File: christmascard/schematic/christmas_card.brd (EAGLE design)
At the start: 50 x 50 mm, 70 parts, among them IC1 WS2811-SOP8, IC2 WS2811-SOP8, IC5 WS2811-SOP8, IC7 74LS595D, U3 ATTINY24/44/84-SSU, X2 USB-MICROB

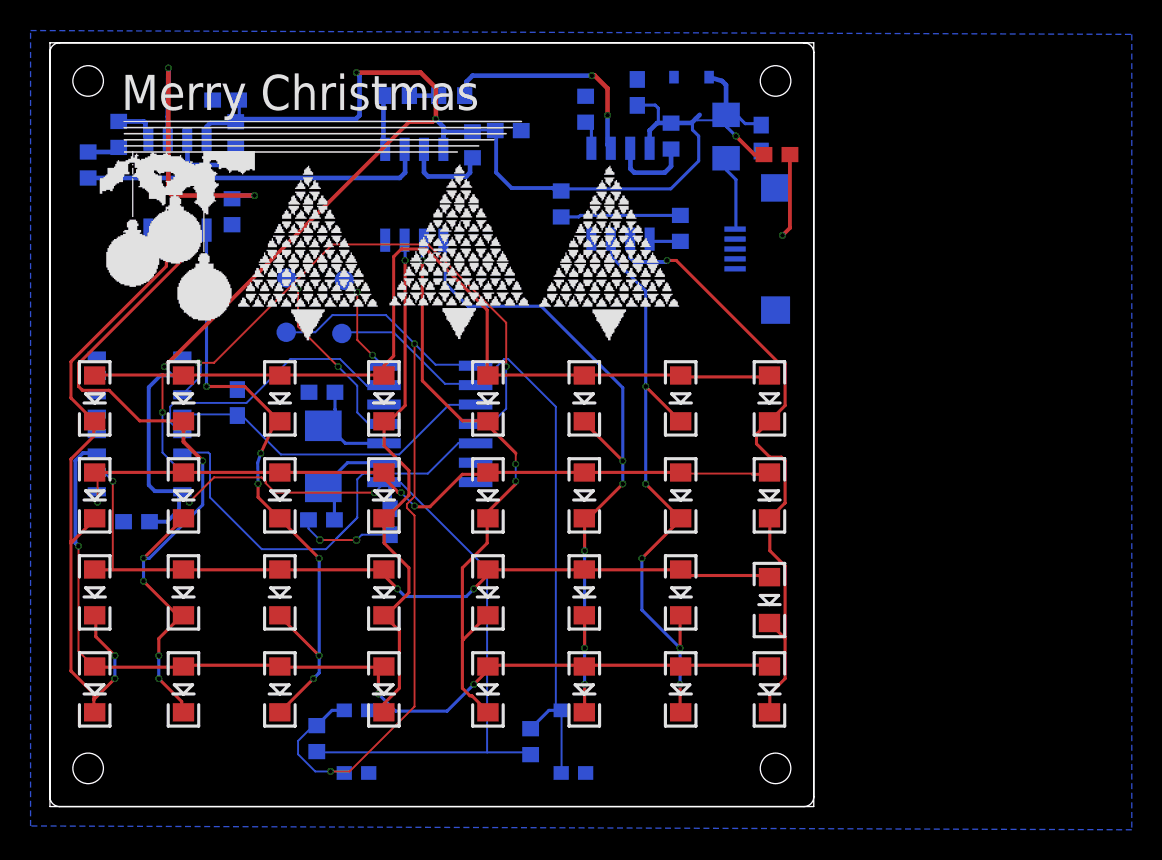
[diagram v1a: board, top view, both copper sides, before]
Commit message: Removed unused files, update board, code and other changes
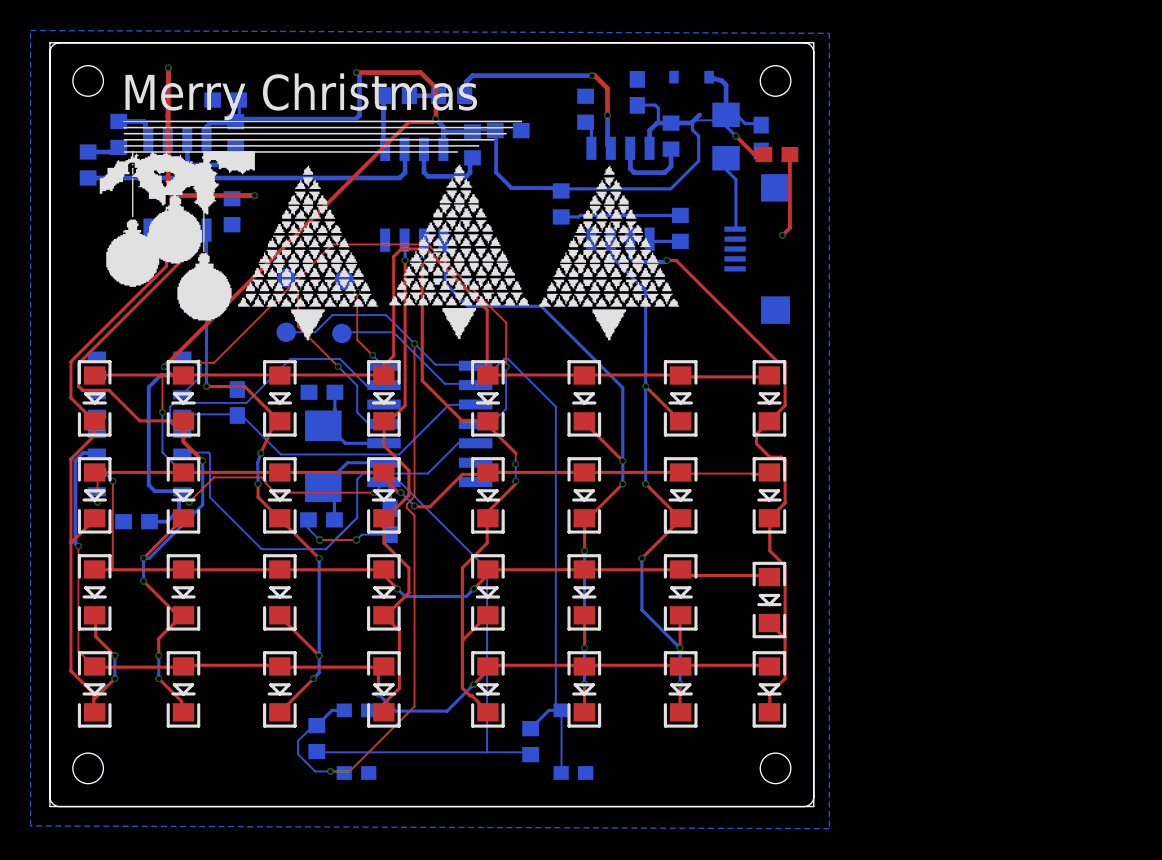
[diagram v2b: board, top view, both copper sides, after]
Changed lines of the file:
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@@
 <drawing>
 <settings>
-<setting alwaysvectorfont="yes"/>
+<setting alwaysvectorfont="no"/>
 <setting keepoldvectorfont="yes"/>
 <setting verticaltext="up"/>
@@
 <polygon width="0.254" layer="16">
 <vertex x="-1.136846875" y="50.751278125"/>
-<vertex x="70.953153125" y="50.501278125"/>
-<vertex x="70.953153125" y="-1.568721875"/>
+<vertex x="51.153153125" y="50.56994375"/>
+<vertex x="51.153153125" y="-1.50005625"/>
 <vertex x="-1.136846875" y="-1.318721875"/>
 </polygon>

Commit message: Improvement and other changes
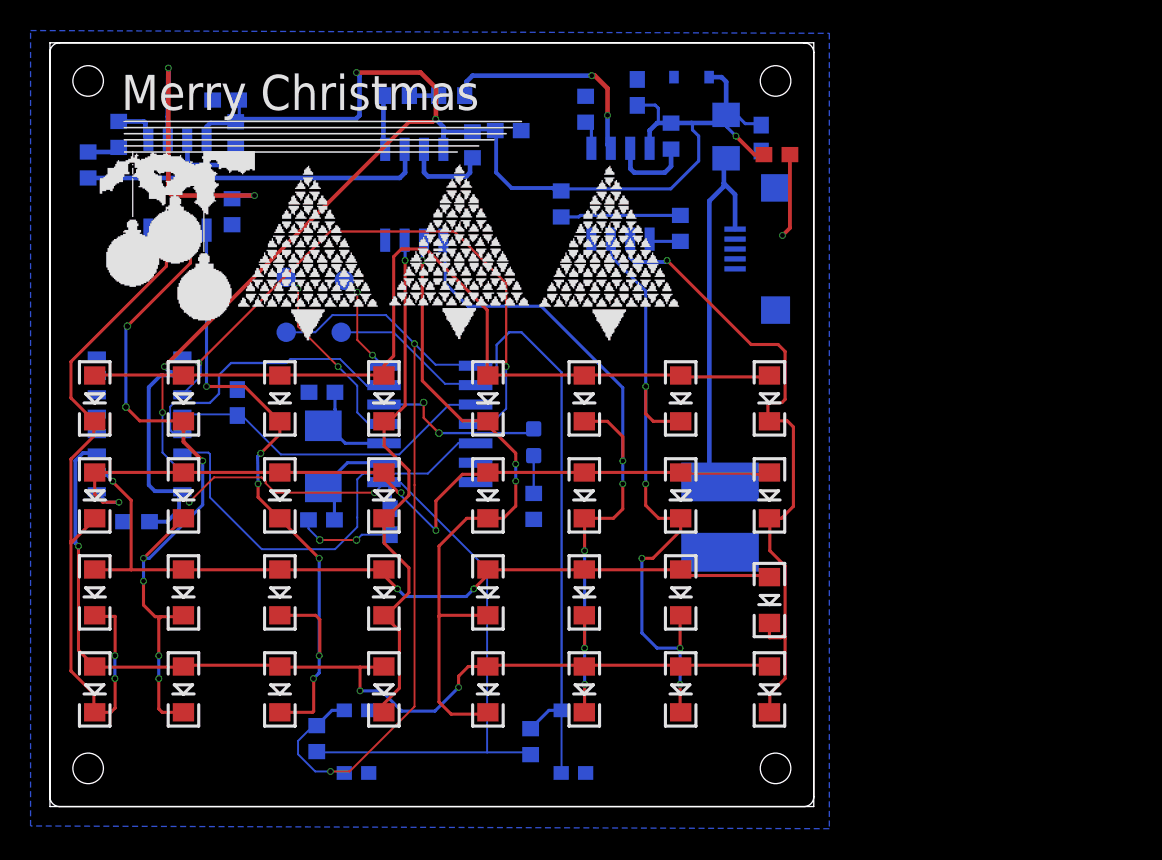
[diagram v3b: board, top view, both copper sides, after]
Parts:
- removed TP1, TP7: TPB1,27, testpad:B1,27
- added 5V, GND: WIREPADSMD2,54-5,08, wirepad:SMD2,54-5,08
- added D2: (no value), SparkFun-LED:LED-0603
- added R4: 480, adafruit:R0603
- added RES, SCK: TPB1,27, testpad:B1,27
- renumbered TP2 to MISO, TP4 to MOSI
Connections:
- removed net N$16: U3.5
- removed net N$41: F1.2, X2.VBUS
- new net DEBUGLED0: D2.A, U3.5
- new net N$9: D2.C, R4.2
- new net VCC: 5V.1, F1.2, X2.VBUS
- net BT0: now also SCK.TP; no longer TP7.TP
- net GND: now also GND.1, R4.1
- net RES: now also RES.TP; no longer TP1.TP
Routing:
- net VCC: track 0.00 -> 25.7 mm
- net DEBUGLED0: track 0.00 -> 11.4 mm, vias 0 -> 2
- net COL4: track 39.8 -> 45.0 mm
- net N$41: track 4.96 -> 0.00 mm
- net LEDROW1: track 49.5 -> 53.9 mm
- net BT0: track 44.2 -> 48.5 mm
- net COL6: track 40.8 -> 44.0 mm
- net COL2: track 42.0 -> 44.9 mm
- net N$9: track 0.00 -> 2.47 mm
- net COL7: track 41.8 -> 44.3 mm
- net COL1: track 49.1 -> 46.8 mm, vias 6 -> 8
- net COL0: track 45.0 -> 47.2 mm
- net RCLK: track 36.1 -> 38.3 mm
- net COL5: track 46.0 -> 47.8 mm
- net SER: track 29.8 -> 28.2 mm
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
